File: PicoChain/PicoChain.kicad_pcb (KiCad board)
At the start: 2 copper layers, 60 x 54 mm, 17 parts, among them J1 RJ45, J2 RJ45, J5 Conn_01x20_Socket, J6 Conn_01x20_Socket, U1 PCA9615DP, U2 RASPBERRY_PI_PICO, U3 LM78M05, U4 LM78M05, U5 LM1085-12

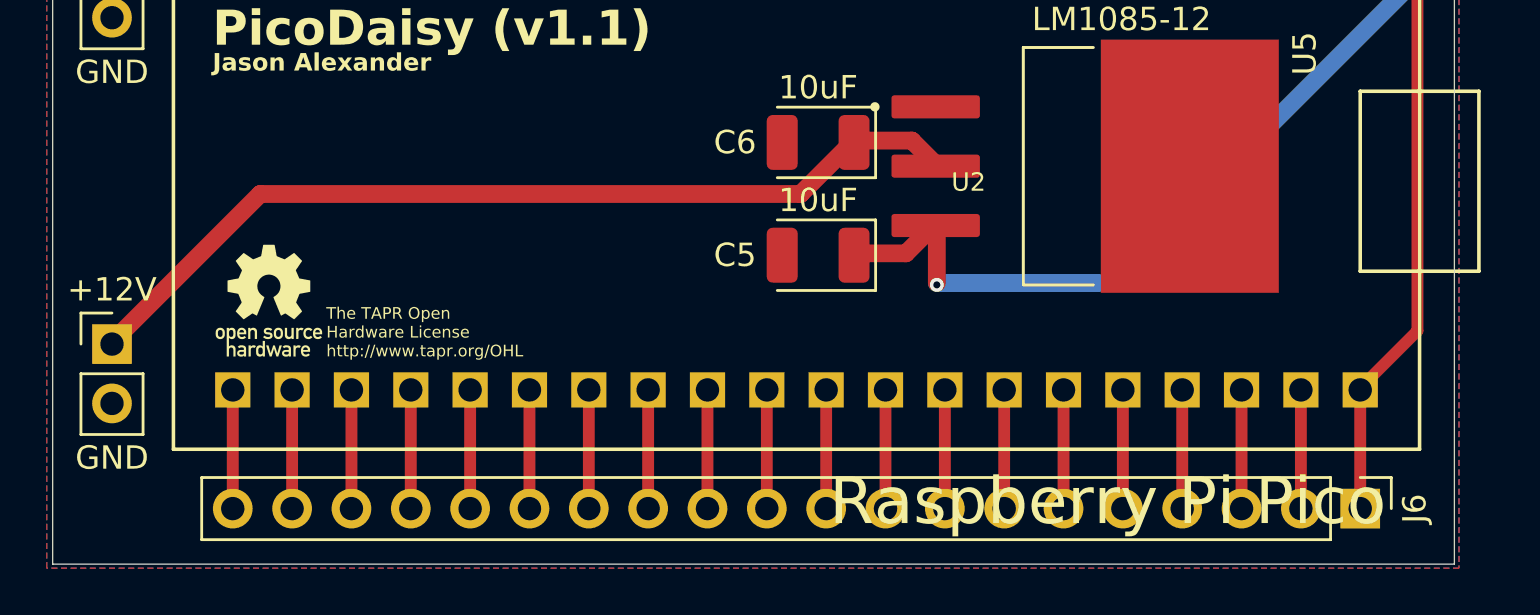
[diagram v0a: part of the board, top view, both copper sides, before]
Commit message: Regenerated gerbers
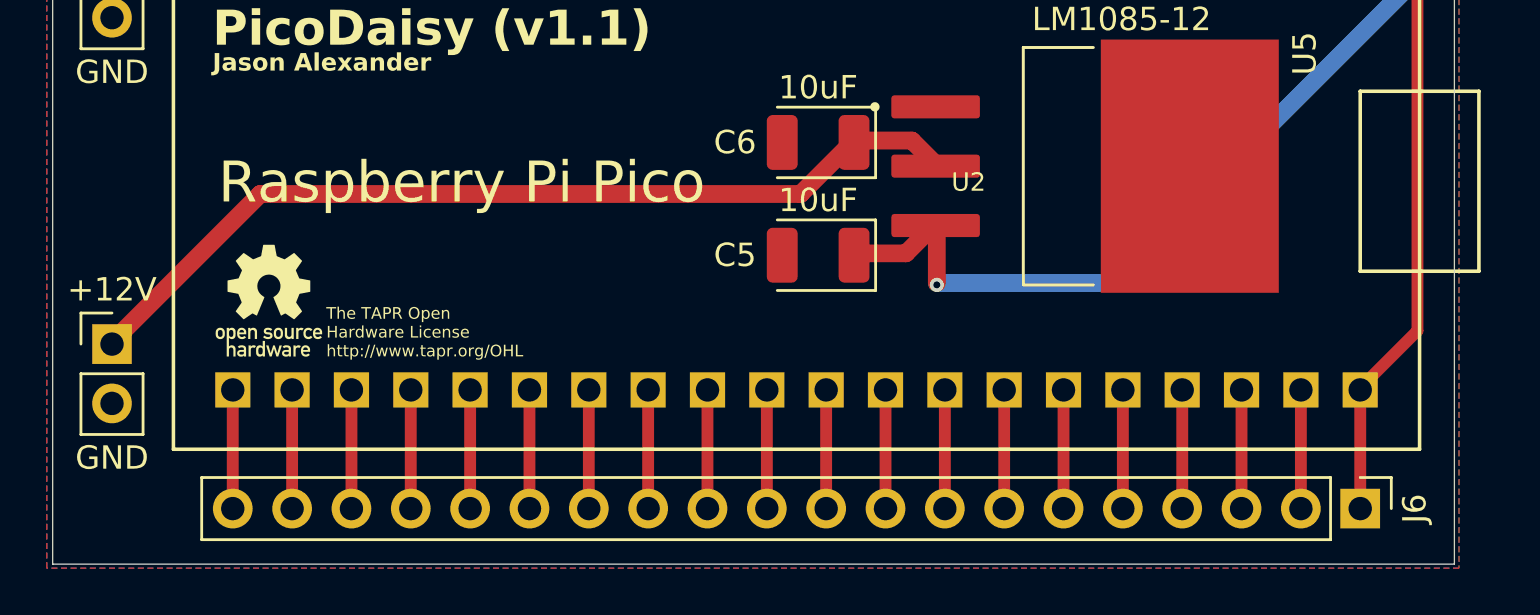
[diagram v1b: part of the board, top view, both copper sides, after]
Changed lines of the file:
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@@
 		)
 		(fp_text user "Raspberry Pi Pico"
-			(at 13.663056 -12.054914 0)
+			(at 0.0114 15.5994 0)
 			(layer "F.SilkS")
 			(effects
 				(font
-					(size 2 2)
+					(size 1.75 1.75)
 					(thickness 0.15)
 				)
